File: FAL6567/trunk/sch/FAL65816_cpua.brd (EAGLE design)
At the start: 100 x 50.8 mm, 18 parts, among them IC12 74LS00D, IC2 74LVC573, IC3 74LS245DW, IC4 74LS688DW, U1 65C816

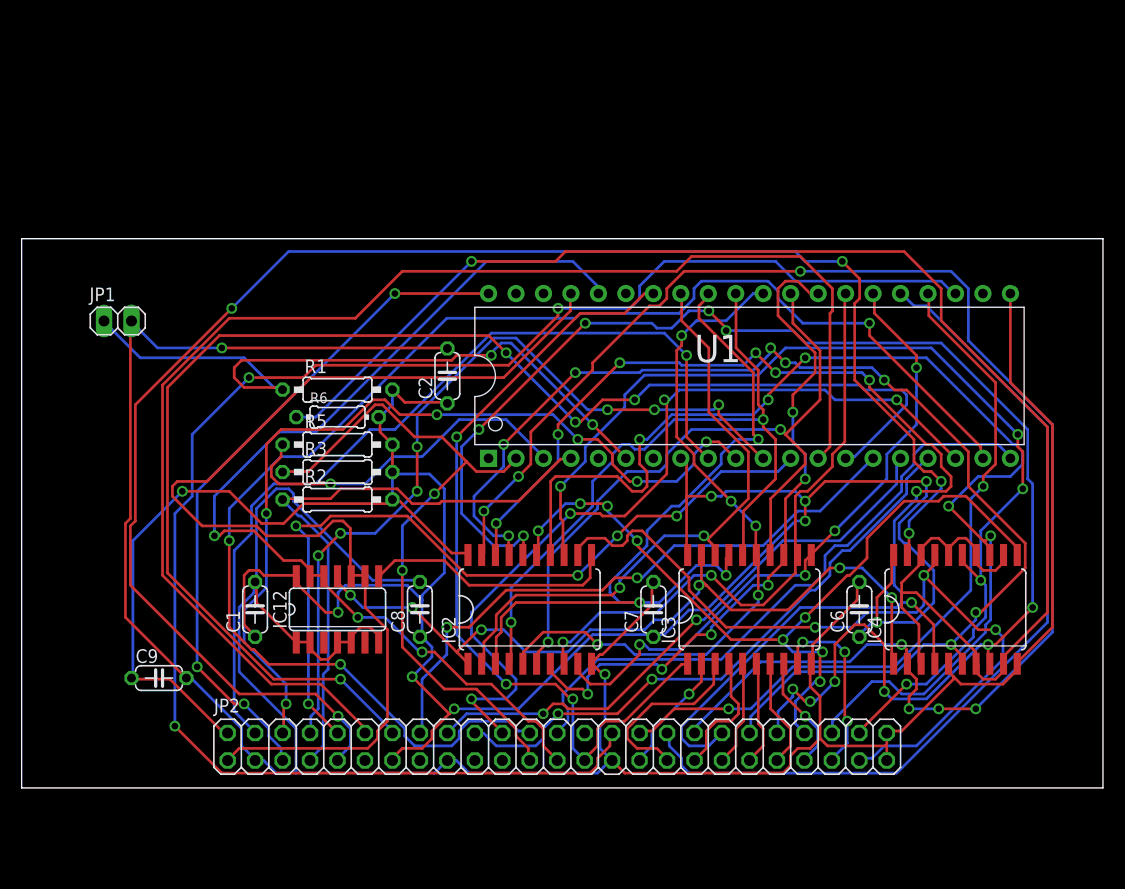
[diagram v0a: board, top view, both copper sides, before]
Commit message: FAL65816 - update
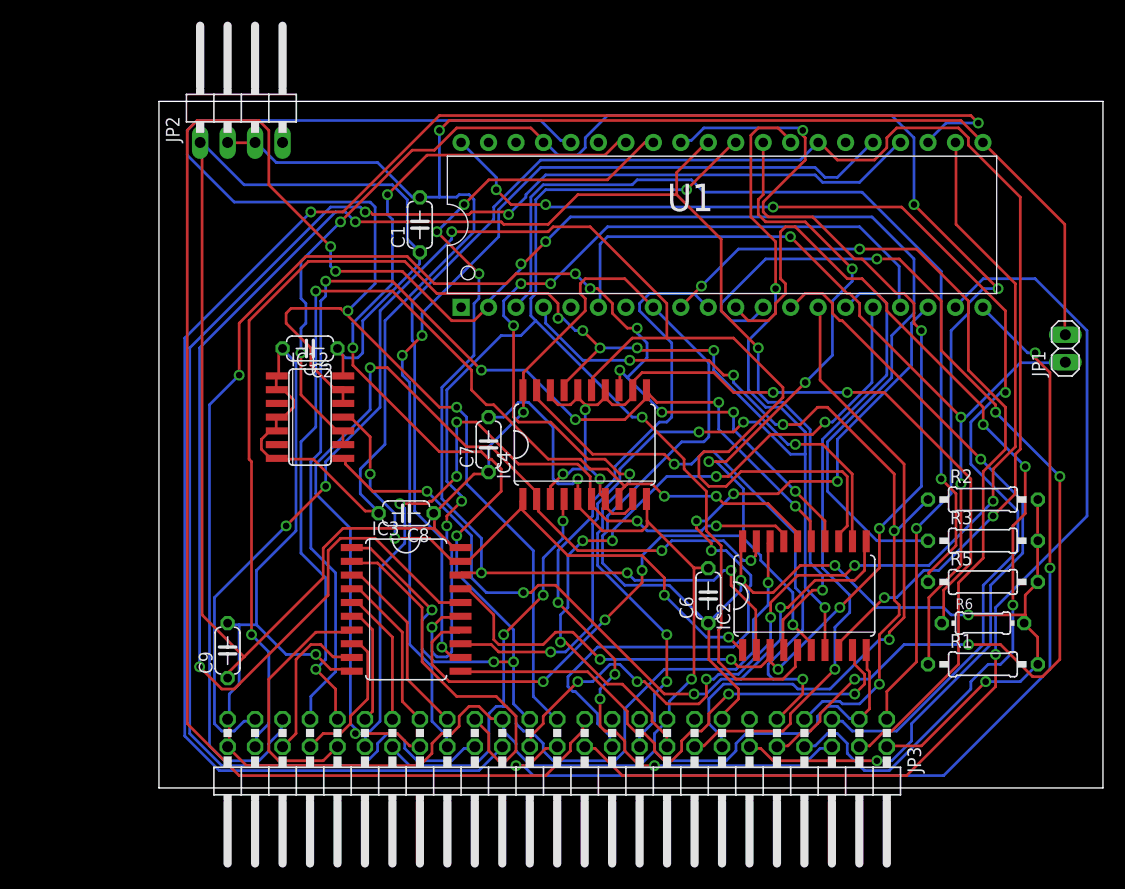
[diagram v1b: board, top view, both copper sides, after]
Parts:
- added JP3: System Bus Conn, pinhead:2X25/90
- JP1: value (none) -> NMI
- JP2: value System Bus Conn -> (none); device pinhead:2X25 -> pinhead:1X04/90
- moved JP1 87.7 mm to (96.5, 40.6), turned to 90 degrees
- moved JP2 66.5 mm to (20.3, 63.5)
- moved R1 64.9 mm to (88.9, 11.4)
- moved R6 62.7 mm to (88.9, 15.2)
- moved R5 61.0 mm to (88.9, 19.1)
- moved R3 60.0 mm to (88.9, 22.9)
- moved R2 59.7 mm to (88.9, 26.7)
- moved C1 38.7 mm to (36.8, 52.1)
- moved IC4 37.5 mm to (52.1, 31.8)
- moved IC3 31.8 mm to (35.6, 16.5), turned to 270 degrees
- moved IC2 25.4 mm to (72.4, 17.8)
- moved C7 21.6 mm to (43.2, 31.8)
- moved IC12 18.0 mm to (26.7, 34.3), turned to 270 degrees
- moved U1 14.2 mm to (63.5, 52.1)
- moved C6 14.0 mm to (63.5, 17.8)
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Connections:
- net N$12 renamed PU1
- net PH2N renamed N$3
- new net +12V: JP2.4
- net A0: now also JP3.4; no longer JP2.4
- net A1: now also JP3.6; no longer JP2.6
- net A10: now also JP3.24; no longer JP2.24
- net A11: now also JP3.26; no longer JP2.26
- net A12: now also JP3.28; no longer JP2.28
- net A13: now also JP3.30; no longer JP2.30
- net A14: now also JP3.32; no longer JP2.32
- net A15: now also JP3.34; no longer JP2.34
- net A16: now also JP3.36; no longer JP2.36
- net A17: now also JP3.38; no longer JP2.38
- net A18: now also JP3.40; no longer JP2.40
- net A19: now also JP3.42; no longer JP2.42
- net A2: now also JP3.8; no longer JP2.8
- net A20: now also JP3.44; no longer JP2.44
- net A21: now also JP3.46; no longer JP2.46
- net A22: now also JP3.48; no longer JP2.48
- net A23: now also JP3.47; no longer JP2.47
- net A3: now also JP3.10; no longer JP2.10
- net A4: now also JP3.12; no longer JP2.12
- net A5: now also JP3.14; no longer JP2.14
- net A6: now also JP3.16; no longer JP2.16
- net A7: now also JP3.18; no longer JP2.18
- net A8: now also JP3.20; no longer JP2.20
- net A9: now also JP3.22; no longer JP2.22
- net AEC: now also JP3.25; no longer JP2.25
- net CLK8: now also JP3.15; no longer JP2.15
- net D7: no longer U1.26
- net GND: now also JP2.2, JP3.17, JP3.29, JP3.3, JP3.49, JP3.50; no longer JP2.17, JP2.29, JP2.49, JP2.50
- net IOSELN: now also JP3.9; no longer JP2.9
- net IRQN: now also JP3.7; no longer JP2.7
- net PH2: now also JP3.1; no longer JP2.1
- net RASN: now also JP3.21; no longer JP2.21
- net RDY: now also JP3.23; no longer JP2.23
- net RESN: now also JP3.5; no longer JP2.5
- net RW: now also JP3.27; no longer JP2.27
- net VCC: now also JP2.1, JP3.13, JP3.2; no longer JP2.13, JP2.2
- net VD0: now also JP3.31; no longer JP2.31
- net VD1: now also JP3.33; no longer JP2.33
- net VD2: now also JP3.35; no longer JP2.35
- net VD3: now also JP3.37; no longer JP2.37
- net VD4: now also JP3.39; no longer JP2.39
- net VD5: now also JP3.41; no longer JP2.41
- net VD6: now also JP3.43; no longer JP2.43
- net VD7: now also JP3.45; no longer JP2.45
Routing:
- net RDY: track 64.0 -> 218.1 mm, vias 2 -> 4
- net D2: track 66.0 -> 172.8 mm, vias 2 -> 4
- net IOSELN: track 150.8 -> 53.5 mm, vias 5 -> 2
- net D6: track 56.9 -> 154.0 mm, vias 2 -> 3
- net A12: track 0.00 -> 95.6 mm, vias 0 -> 6
- net A14: track 67.2 -> 142.0 mm
- net A5: track 128.2 -> 58.9 mm, vias 4 -> 1
- net PU1: track 147.6 -> 83.0 mm, vias 1 -> 5
- net D3: track 63.6 -> 125.4 mm
- net A4: track 127.0 -> 73.2 mm, vias 0 -> 2
- net A16: track 142.3 -> 90.2 mm, vias 7 -> 4
- net ABORTN: track 32.8 -> 83.2 mm
- net RESN: track 63.2 -> 110.9 mm, vias 3 -> 4
- net GND: track 299.5 -> 347.0 mm, vias 2 -> 4
- net A23: track 73.4 -> 120.3 mm, vias 3 -> 7
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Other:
- board size 100 x 50.8 mm -> 87.3 x 63.5 mm
